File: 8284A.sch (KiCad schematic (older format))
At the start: 6 parts, among them SW22 SW_Push, U27 8284, Y1 15MHz

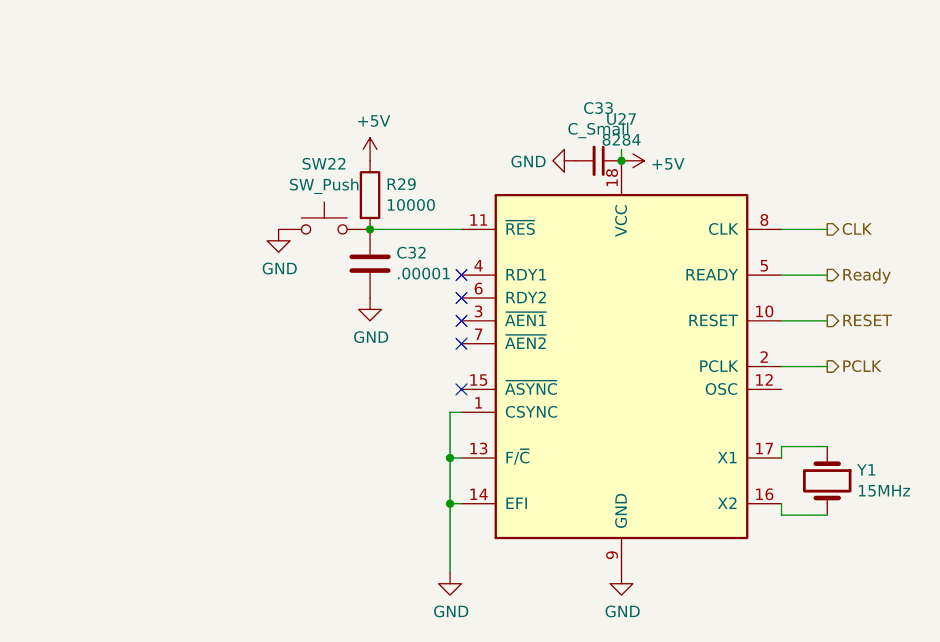
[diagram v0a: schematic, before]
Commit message: Fixing Weirdness
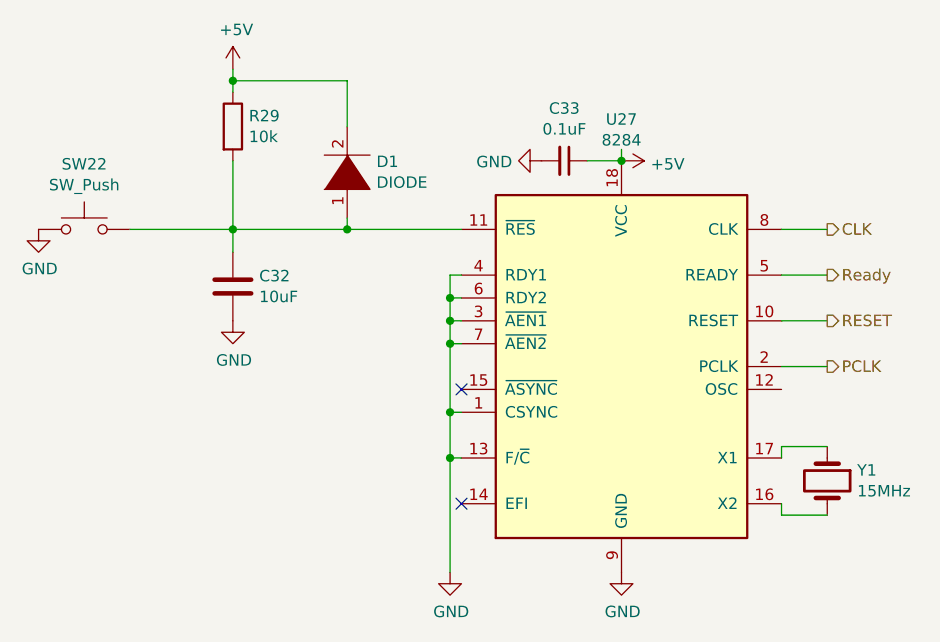
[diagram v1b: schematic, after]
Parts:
- added D1: DIODE, symbol pspice:DIODE
- C32: value .00001 -> 10uF
- C33: value C_Small -> 0.1uF
- R29: value 10000 -> 10k
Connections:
- wire segments 16 -> 32
- no-connect marks 5 -> 2
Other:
- moved on the sheet: C32, C33, R29, SW22
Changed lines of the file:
@@
 	0    1    1    0
 $EndComp
+Wire Wire Line
+	5650 2200 5650 2250
+Connection ~ 5650 2250
+Wire Wire Line
+	6350 2550 6550 2550
+Wire Wire Line
+	6350 2950 6550 2950
+Wire Wire Line
+	6350 3150 6550 3150
+$Comp
+L Device:Crystal Y1
+U 1 1 61C4A363
+P 6550 3650
+F 0 "Y1" V 6504 3781 50  0000 L CNN
+F 1 "15MHz" V 6595 3781 50  0000 L CNN
+F 2 "" H 6550 3650 50  0001 C CNN
+F 3 "~" H 6550 3650 50  0001 C CNN
+	1    6550 3650
+	0    1    1    0
+$EndComp
+Wire Wire Line
+	6350 3550 6350 3500
+Wire Wire Line
+	6350 3500 6550 3500
+Wire Wire Line
+	6350 3750 6350 3800
+Wire Wire Line
+	6350 3800 6550 3800
+Wire Wire Line
+	4950 3350 4900 3350
+Wire Wire Line
+	4900 3350 4900 3550
+$Comp
+L power:GND #PWR0126
+U 1 1 61C4C338
+P 4900 4050
+F 0 "#PWR0126" H 4900 3800 50  0001 C CNN
+F 1 "GND" H 4905 3877 50  0000 C CNN
+F 2 "" H 4900 4050 50  0001 C CNN
+F 3 "" H 4900 4050 50  0001 C CNN
+	1    4900 4050
+	1    0    0    -1
+$EndComp
+Wire Wire Line
+	4950 3550 4900 3550
+Connection ~ 4900 3550
+NoConn ~ 4950 3250
+$Comp
+L Device:R R29
+U 1 1 61C4FCA9
+P 3950 2100
+F 0 "R29" H 4020 2146 50  0000 L CNN
+F 1 "10k" H 4020 2055 50  0000 L CNN
+F 2 "" V 3880 2100 50  0001 C CNN
+F 3 "~" H 3950 2100 50  0001 C CNN
+	1    3950 2100
+	1    0    0    -1
+$EndComp
+$Comp
+L Device:C C32
+U 1 1 61C51F9B
+P 3950 2800
+F 0 "C32" H 4065 2846 50  0000 L CNN
+F 1 "10uF" H 4065 2755 50  0000 L CNN
+F 2 "" H 3988 2650 50  0001 C CNN
+F 3 "~" H 3950 2800 50  0001 C CNN
+	1    3950 2800
+	1    0    0    -1
+$EndComp
+$Comp
+L power:GND #PWR0127
+U 1 1 61C52E7D
+P 3950 2950
+F 0 "#PWR0127" H 3950 2700 50  0001 C CNN
+F 1 "GND" H 3955 2777 50  0000 C CNN
+F 2 "" H 3950 2950 50  0001 C CNN
+F 3 "" H 3950 2950 50  0001 C CNN
+	1    3950 2950
+	1    0    0    -1
+$EndComp
+$Comp
+L power:+5V #PWR0128
+U 1 1 61C55057
+P 3950 1850
+F 0 "#PWR0128" H 3950 1700 50  0001 C CNN
+F 1 "+5V" H 3965 2023 50  0000 C CNN
+F 2 "" H 3950 1850 50  0001 C CNN
+F 3 "" H 3950 1850 50  0001 C CNN
+	1    3950 1850
+	1    0    0    -1
+$EndComp
+$Comp
+L Switch:SW_Push SW22
+U 1 1 61C5620F
+P 3300 2550
+F 0 "SW22" H 3300 2835 50  0000 C CNN
+F 1 "SW_Push" H 3300 2744 50  0000 C CNN
+F 2 "" H 3300 2750 50  0001 C CNN
+F 3 "~" H 3300 2750 50  0001 C CNN
+	1    3300 2550
+	1    0    0    -1
+$EndComp
+$Comp
+L power:GND #PWR0129
+U 1 1 61C57263
+P 3100 2550
+F 0 "#PWR0129" H 3100 2300 50  0001 C CNN
+F 1 "GND" H 3105 2377 50  0000 C CNN
+F 2 "" H 3100 2550 50  0001 C CNN
+F 3 "" H 3100 2550 50  0001 C CNN
+	1    3100 2550
+	1    0    0    -1
+$EndComp
+Text HLabel 6550 2550 2    50   Output ~ 0
+CLK
+Text HLabel 6550 2950 2    50   Output ~ 0
+RESET
+Text HLabel 6550 3150 2    50   Output ~ 0
+PCLK
+$Comp
+L Device:C_Small C33
+U 1 1 61F73A25
+P 5400 2250
+F 0 "C33" V 5171 2250 50  0000 C CNN
+F 1 "0.1uF" V 5262 2250 50  0000 C CNN
+F 2 "" H 5400 2250 50  0001 C CNN
+F 3 "~" H 5400 2250 50  0001 C CNN
+	1    5400 2250
+	0    1    1    0
+$EndComp
+$Comp
+L power:GND #PWR0130
+U 1 1 61F73F55
+P 5300 2250
+F 0 "#PWR0130" H 5300 2000 50  0001 C CNN
+F 1 "GND" V 5305 2122 50  0000 R CNN
+F 2 "" H 5300 2250 50  0001 C CNN
+F 3 "" H 5300 2250 50  0001 C CNN
+	1    5300 2250
+	0    1    1    0
+$EndComp
+Wire Wire Line
+	6350 2750 6550 2750
+Text HLabel 6550 2750 2    50   Output ~ 0
+Ready
 $Comp
 L Timer:8284 U27
@@
 $EndComp
 Wire Wire Line
-	5650 2200 5650 2250
-Connection ~ 5650 2250
-Wire Wire Line
-	6350 2550 6550 2550
-Wire Wire Line
-	6350 2950 6550 2950
-Wire Wire Line
-	6350 3150 6550 3150
-$Comp
-L Device:Crystal Y1
-U 1 1 61C4A363
-P 6550 3650
-F 0 "Y1" V 6504 3781 50  0000 L CNN
-F 1 "15MHz" V 6595 3781 50  0000 L CNN
-F 2 "" H 6550 3650 50  0001 C CNN
-F 3 "~" H 6550 3650 50  0001 C CNN
-	1    6550 3650
-	0    1    1    0
-$EndComp
-Wire Wire Line
-	6350 3550 6350 3500
-Wire Wire Line
-	6350 3500 6550 3500
-Wire Wire Line
-	6350 3750 6350 3800
-Wire Wire Line
-	6350 3800 6550 3800
-Wire Wire Line
-	4950 3350 4900 3350
-Wire Wire Line
-	4900 3350 4900 3550
-$Comp
-L power:GND #PWR0126
-U 1 1 61C4C338
-P 4900 4050
-F 0 "#PWR0126" H 4900 3800 50  0001 C CNN
-F 1 "GND" H 4905 3877 50  0000 C CNN
-F 2 "" H 4900 4050 50  0001 C CNN
-F 3 "" H 4900 4050 50  0001 C CNN
-	1    4900 4050
-	1    0    0    -1
-$EndComp
-Wire Wire Line
-	4950 3550 4900 3550
-Connection ~ 4900 3550
-Wire Wire Line
-	4900 3550 4900 3750
-Wire Wire Line
-	4900 3750 4950 3750
-Connection ~ 4900 3750
-Wire Wire Line
-	4900 3750 4900 4050
-NoConn ~ 4950 3250
-NoConn ~ 4950 2750
-NoConn ~ 4950 2850
-NoConn ~ 4950 2950
-NoConn ~ 4950 3050
-$Comp
-L Device:R R29
-U 1 1 61C4FCA9
-P 4550 2400
-F 0 "R29" H 4620 2446 50  0000 L CNN
-F 1 "10000" H 4620 2355 50  0000 L CNN
-F 2 "" V 4480 2400 50  0001 C CNN
-F 3 "~" H 4550 2400 50  0001 C CNN
-	1    4550 2400
-	1    0    0    -1
-$EndComp
-$Comp
-L Device:C C32
-U 1 1 61C51F9B
-P 4550 2700
-F 0 "C32" H 4665 2746 50  0000 L CNN
-F 1 ".00001" H 4665 2655 50  0000 L CNN
-F 2 "" H 4588 2550 50  0001 C CNN
-F 3 "~" H 4550 2700 50  0001 C CNN
-	1    4550 2700
-	1    0    0    -1
-$EndComp
-$Comp
-L power:GND #PWR0127
-U 1 1 61C52E7D
-P 4550 2850
-F 0 "#PWR0127" H 4550 2600 50  0001 C CNN
-F 1 "GND" H 4555 2677 50  0000 C CNN
-F 2 "" H 4550 2850 50  0001 C CNN
-F 3 "" H 4550 2850 50  0001 C CNN
-	1    4550 2850
-	1    0    0    -1
-$EndComp
-Connection ~ 4550 2550
-Wire Wire Line
-	4550 2550 4950 2550
-$Comp
-L power:+5V #PWR0128
-U 1 1 61C55057
-P 4550 2250
-F 0 "#PWR0128" H 4550 2100 50  0001 C CNN
-F 1 "+5V" H 4565 2423 50  0000 C CNN
-F 2 "" H 4550 2250 50  0001 C CNN
-F 3 "" H 4550 2250 50  0001 C CNN
-	1    4550 2250
-	1    0    0    -1
-$EndComp
-$Comp
-L Switch:SW_Push SW22
-U 1 1 61C5620F
-P 4350 2550
-F 0 "SW22" H 4350 2835 50  0000 C CNN
-F 1 "SW_Push" H 4350 2744 50  0000 C CNN
-F 2 "" H 4350 2750 50  0001 C CNN
-F 3 "~" H 4350 2750 50  0001 C CNN
-	1    4350 2550
-	1    0    0    -1
-$EndComp
-$Comp
-L power:GND #PWR0129
-U 1 1 61C57263
-P 4150 2550
-F 0 "#PWR0129" H 4150 2300 50  0001 C CNN
-F 1 "GND" H 4155 2377 50  0000 C CNN
-F 2 "" H 4150 2550 50  0001 C CNN
-F 3 "" H 4150 2550 50  0001 C CNN
-	1    4150 2550
-	1    0    0    -1
-$EndComp
-Text HLabel 6550 2550 2    50   Output ~ 0
-CLK
-Text HLabel 6550 2950 2    50   Output ~ 0
-RESET
-Text HLabel 6550 3150 2    50   Output ~ 0
-PCLK
-$Comp
-L Device:C_Small C33
-U 1 1 61F73A25
-P 5550 2250
-F 0 "C33" V 5321 2250 50  0000 C CNN
-F 1 "C_Small" V 5412 2250 50  0000 C CNN
-F 2 "" H 5550 2250 50  0001 C CNN
-F 3 "~" H 5550 2250 50  0001 C CNN
-	1    5550 2250
-	0    1    1    0
-$EndComp
-$Comp
-L power:GND #PWR0130
-U 1 1 61F73F55
-P 5450 2250
-F 0 "#PWR0130" H 5450 2000 50  0001 C CNN
-F 1 "GND" V 5455 2122 50  0000 R CNN
-F 2 "" H 5450 2250 50  0001 C CNN
-F 3 "" H 5450 2250 50  0001 C CNN
-	1    5450 2250
-	0    1    1    0
-$EndComp
-Wire Wire Line
-	6350 2750 6550 2750
-Text HLabel 6550 2750 2    50   Output ~ 0
-Ready
+	4900 3350 4900 3050
+Wire Wire Line
+	4900 2750 4950 2750
+Connection ~ 4900 3350
+Wire Wire Line
+	4950 2850 4900 2850
+Connection ~ 4900 2850
+Wire Wire Line
+	4900 2850 4900 2750
+Wire Wire Line
+	4900 2950 4950 2950
+Connection ~ 4900 2950
+Wire Wire Line
+	4900 2950 4900 2850
+Wire Wire Line
+	4900 3050 4950 3050
+Connection ~ 4900 3050
+Wire Wire Line
+	4900 3050 4900 2950
+Wire Wire Line
+	3950 1850 3950 1900
+Wire Wire Line
+	3950 2250 3950 2550
+Wire Wire Line
+	3950 2650 3950 2550
+Connection ~ 3950 2550
+Wire Wire Line
+	3500 2550 3950 2550
+Wire Wire Line
+	3950 2550 4450 2550
+$Comp
+L pspice:DIODE D1
+U 1 1 61B9009B
+P 4450 2300
+F 0 "D1" V 4496 2172 50  0000 R CNN
+F 1 "DIODE" V 4405 2172 50  0000 R CNN
+F 2 "" H 4450 2300 50  0001 C CNN
+F 3 "~" H 4450 2300 50  0001 C CNN
+	1    4450 2300
+	0    -1   -1   0
+$EndComp
+Wire Wire Line
+	4450 2550 4450 2500
+Connection ~ 4450 2550
+Wire Wire Line
+	4450 2550 4950 2550
+Wire Wire Line
+	4450 2100 4450 1900
+Wire Wire Line
+	4450 1900 3950 1900
+Connection ~ 3950 1900
+Wire Wire Line
+	3950 1900 3950 1950
+Wire Wire Line
+	4900 3550 4900 4050
+NoConn ~ 4950 3750
+Wire Wire Line
+	5650 2250 5500 2250
 $EndSCHEMATC
